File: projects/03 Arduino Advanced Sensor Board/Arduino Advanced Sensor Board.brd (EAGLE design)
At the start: 68.6 x 53.3 mm, 53 parts

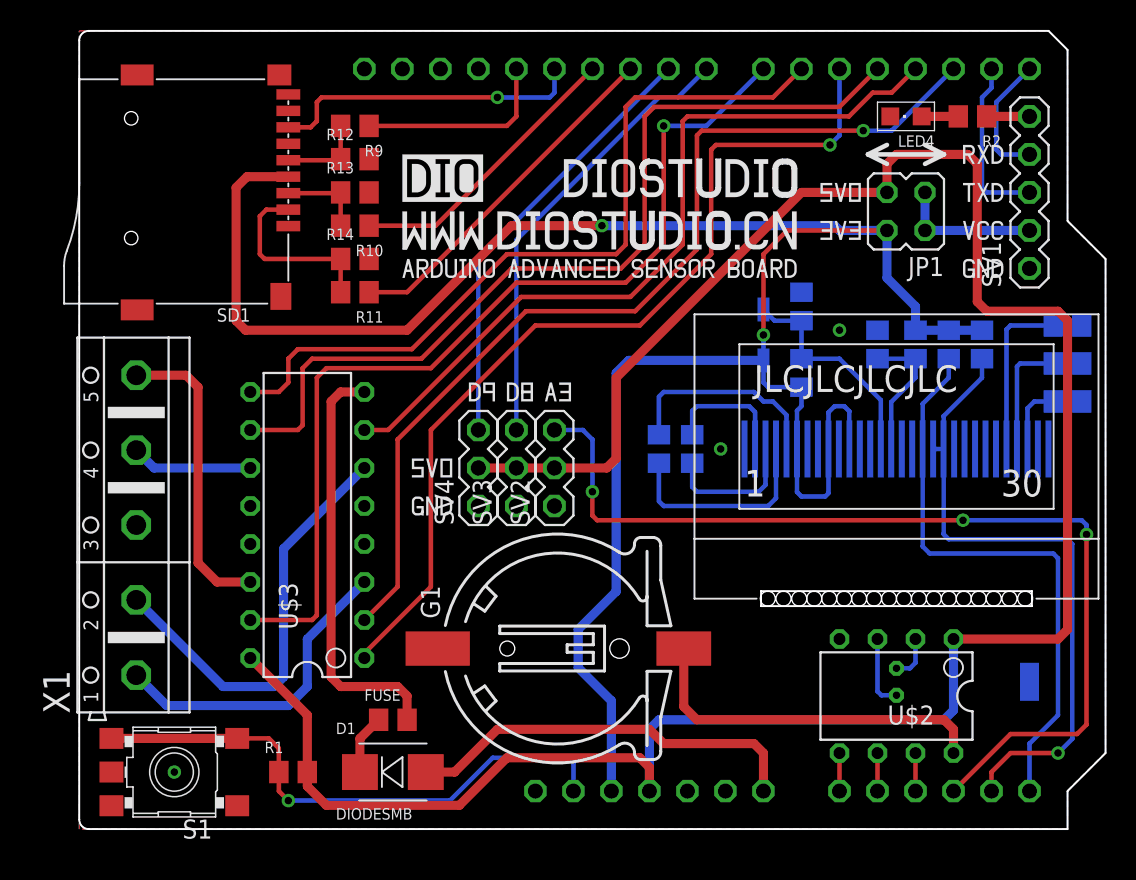
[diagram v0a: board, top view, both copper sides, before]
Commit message: 2020.07.01.01
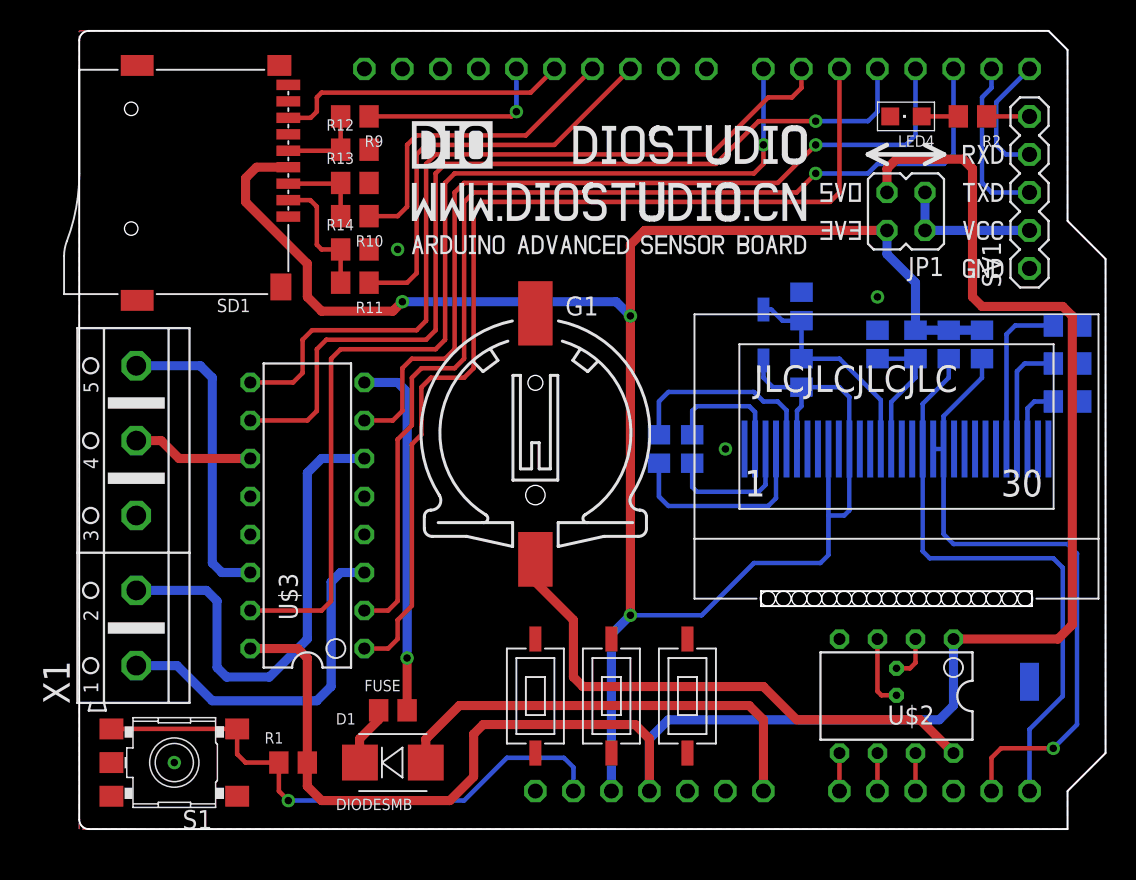
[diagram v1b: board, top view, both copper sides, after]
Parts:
- removed SV2, SV3, SV4: (no value), Pin-Header:MA03-1
- removed U$18: (no value), Logos:D8_050
- removed U$19: (no value), Logos:D9_050
- removed U$20: (no value), Logos:5V0_050
- removed U$21: (no value), Logos:GND_050
- removed U$22: (no value), Logos:A3_050
- added U$23, U$24, U$25: (no value), Button:TS-SMD_3*6
- U$14: device Logos:DIOSTUDIO_100 -> Logos:LOGO_100
- U$15: device Logos:LOGO_100 -> Logos:WWW.DIOSTUDIO.CN_100
- U$16: device Logos:WWW.DIOSTUDIO.CN_100 -> Logos:DIOSTUDIO_100
- moved U$16 12.8 mm to (33.0, 44.5)
- moved G1 11.2 mm to (30.5, 20.3), turned to 0 degrees
- moved U$14 10.3 mm to (22.2, 44.1)
- moved U$17 7.30 mm to (44.8, 37.1)
- moved U$13 1.71 mm to (22.2, 38.4)
- moved U$15 1.42 mm to (22.2, 40.6)
- moved R10 0.64 mm to (18.4, 41.0)
- moved R11 0.64 mm to (18.4, 36.5)
- moved R12 0.64 mm to (18.4, 45.4)
- moved D1 0.64 mm to (21.0, 4.45)
- moved R1 0.64 mm to (14.3, 4.45)
- moved S1 0.64 mm to (6.35, 4.45)
- moved FUSE 0.63 mm to (21.0, 7.94)
- moved R13 0.63 mm to (18.4, 43.2)
- moved R14 0.63 mm to (18.4, 38.7)
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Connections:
- net 5V0: no longer SV2.2, SV3.2, SV4.2
- net A3: no longer SV2.3
- net D8: no longer SV3.3
- net D9: no longer SV4.3
- net GND: no longer SV2.1, SV3.1, SV4.1
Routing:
- net A3: track 65.2 -> 0.00 mm, vias 3 -> 0
- net 5V0: track 157.3 -> 125.3 mm
- net D8: track 30.1 -> 0.00 mm
- net D9: track 29.4 -> 0.00 mm
- net N$6: track 24.1 -> 36.4 mm
- net IN1: track 64.9 -> 72.0 mm
- net PWM1: track 61.1 -> 67.7 mm, vias 1 -> 0
- net 3V3: track 150.7 -> 144.7 mm, vias 2 -> 3
- net IN2: track 51.7 -> 57.0 mm, vias 0 -> 1
- net IN4: track 63.5 -> 68.6 mm
- net SS: track 23.6 -> 28.0 mm
- net OUT2: track 28.7 -> 32.8 mm
- net N$9: track 12.4 -> 8.57 mm
- net VCC: track 28.1 -> 24.4 mm, vias 0 -> 1
- net VIN: track 26.9 -> 30.2 mm
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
